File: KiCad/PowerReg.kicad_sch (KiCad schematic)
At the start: 4 parts, among them U2 TPS62162DSG

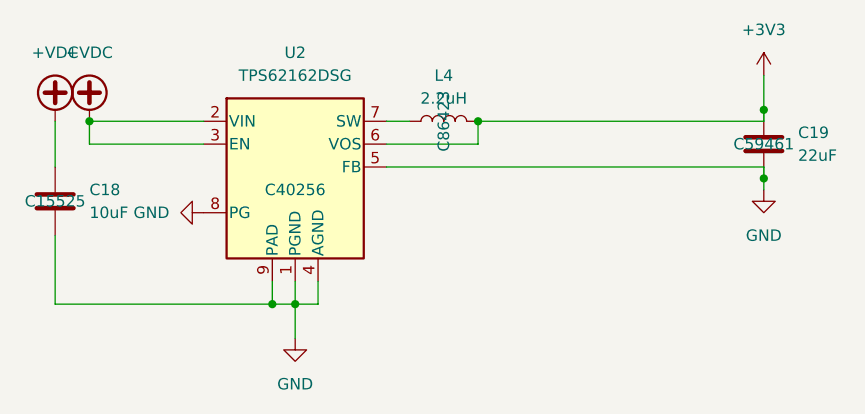
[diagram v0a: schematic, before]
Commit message: fixed a couple issues
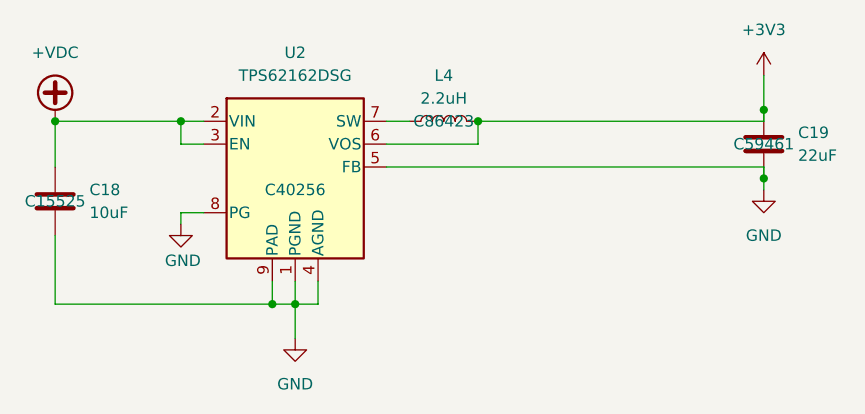
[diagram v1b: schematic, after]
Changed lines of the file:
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@@
 	(paper "A4")
+	(junction
+		(at 110.49 57.15)
+		(diameter 0)
+		(color 0 0 0 0)
+	)
 	(junction
 		(at 123.19 77.47)
@@
 	)
 	(junction
+		(at 96.52 57.15)
+		(diameter 0)
+		(color 0 0 0 0)
+	)
+	(junction
 		(at 175.26 55.88)
 		(diameter 0)
 		(color 0 0 0 0)
 	)
-	(junction
-		(at 100.33 57.15)
-		(diameter 0)
-		(color 0 0 0 0)
-	)
 	(wire
 		(pts
@@
 	(wire
 		(pts
-			(xy 100.33 59.69) (xy 113.03 59.69)
-		)
-		(stroke
-			(width 0)
-			(type default)
-		)
-	)
-	(wire
-		(pts
 			(xy 123.19 74.93) (xy 123.19 77.47)
 		)
@@
 	(wire
 		(pts
+			(xy 110.49 67.31) (xy 110.49 68.58)
+		)
+		(stroke
+			(width 0)
+			(type default)
+		)
+	)
+	(wire
+		(pts
 			(xy 175.26 62.23) (xy 175.26 63.5)
 		)
@@
 	(wire
 		(pts
-			(xy 100.33 57.15) (xy 100.33 59.69)
+			(xy 113.03 59.69) (xy 110.49 59.69)
 		)
 		(stroke
@@
 	(wire
 		(pts
+			(xy 110.49 57.15) (xy 113.03 57.15)
+		)
+		(stroke
+			(width 0)
+			(type default)
+		)
+	)
+	(wire
+		(pts
 			(xy 143.51 57.15) (xy 143.51 59.69)
 		)
@@
 	(wire
 		(pts
-			(xy 100.33 57.15) (xy 113.03 57.15)
+			(xy 110.49 67.31) (xy 113.03 67.31)
+		)
+		(stroke
+			(width 0)
+			(type default)
+		)
+	)
+	(wire
+		(pts
+			(xy 96.52 57.15) (xy 110.49 57.15)
+		)
+		(stroke
+			(width 0)
+			(type default)
+		)
+	)
+	(wire
+		(pts
+			(xy 110.49 59.69) (xy 110.49 57.15)
 		)
 		(stroke
@@
 	(symbol
 		(lib_id "power:GND")
-		(at 113.03 67.31 270)
+		(at 110.49 68.58 0)
 		(unit 1)
 		(exclude_from_sim no)
@@
 		(on_board yes)
 		(dnp no)
-		(fields_autoplaced yes)
 		(property "Reference" "#PWR040"
-			(at 106.68 67.31 0)
+			(at 110.49 74.93 0)
 			(effects
 				(font
@@
 		)
 		(property "Value" "GND"
-			(at 109.22 67.3099 90)
-			(effects
-				(font
-					(size 1.27 1.27)
-				)
-				(justify right)
+			(at 108.712 72.644 0)
+			(effects
+				(font
+					(size 1.27 1.27)
+				)
+				(justify left)
 			)
 		)
 		(property "Footprint" ""
-			(at 113.03 67.31 0)
+			(at 110.49 68.58 0)
 			(effects
 				(font
@@
 		)
 		(property "Datasheet" ""
-			(at 113.03 67.31 0)
+			(at 110.49 68.58 0)
 			(effects
 				(font
@@
 		)
 		(property "Description" "Power symbol creates a global label with name \"GND\" , ground"
-			(at 113.03 67.31 0)
+			(at 110.49 68.58 0)
 			(effects
 				(font
@@
 		(on_board yes)
 		(dnp no)
-		(fields_autoplaced yes)
 		(property "Reference" "L4"
 			(at 139.7 52.07 90)
@@
 		)
 		(property "LCSC" "C86423"
-			(at 139.7 57.15 0)
+			(at 139.7 57.15 90)
 			(effects
 				(font
@@
 					(unit 1)
 				)
-			)
-		)
-	)
-	(symbol
-		(lib_id "power:+VDC")
-		(at 100.33 57.15 0)
-		(unit 1)
-		(exclude_from_sim no)
-		(in_bom yes)
-		(on_board yes)
-		(dnp no)
-		(fields_autoplaced yes)
-		(property "Reference" "#PWR034"
-			(at 100.33 59.69 0)
-			(effects
-				(font
-					(size 1.27 1.27)
-				)
-				(hide yes)
-			)
-		)
-		(property "Value" "+VDC"
-			(at 100.33 49.53 0)
-			(effects
-				(font
-					(size 1.27 1.27)
-				)
-			)
-		)
-		(property "Footprint" ""
-			(at 100.33 57.15 0)
-			(effects
-				(font
-					(size 1.27 1.27)
-				)
-				(hide yes)
-			)
-		)
-		(property "Datasheet" ""
-			(at 100.33 57.15 0)
-			(effects
-				(font
-					(size 1.27 1.27)
-				)
-				(hide yes)
-			)
-		)
-		(property "Description" "Power symbol creates a global label with name \"+VDC\""
-			(at 100.33 57.15 0)
-			(effects
-				(font
-					(size 1.27 1.27)
-				)
-				(hide yes)
-			)
-		)
-		(pin "1"
-		)
-		(instances
-			(project ""
-				(path "/16f8cce7-467e-4342-b55a-00af81cd6f69/bf62daab-1cf5-4742-a85c-ffd3166ecdf9"
-					(reference "#PWR034")
-					(unit 1)
-				)
